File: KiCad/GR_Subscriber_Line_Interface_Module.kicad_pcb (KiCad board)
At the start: 2 copper layers, 99.3 x 99.5 mm, 112 parts, among them J1 Conn_01x03, J10 PJ-202A, J11 Screw_Terminal_01x02, J2 Conn_01x08, J3 Jumper, J4 Conn_01x06, J5 Conn_01x02, J6 RJ, J7 RJ, J8 Conn_01x03, J9 Jumper, K1 HK19F-DC5V-SHG, Q1 2N7000, Q2 2N3904, T1 600:600, U1 ESP32_DevKit_V1_DOIT, U2 MT8870DE, U3 4050, U4 KS0835F, U5 LM358, U6 LD1117AV33, U7 ICL7660, Y1 3.579545 MHz

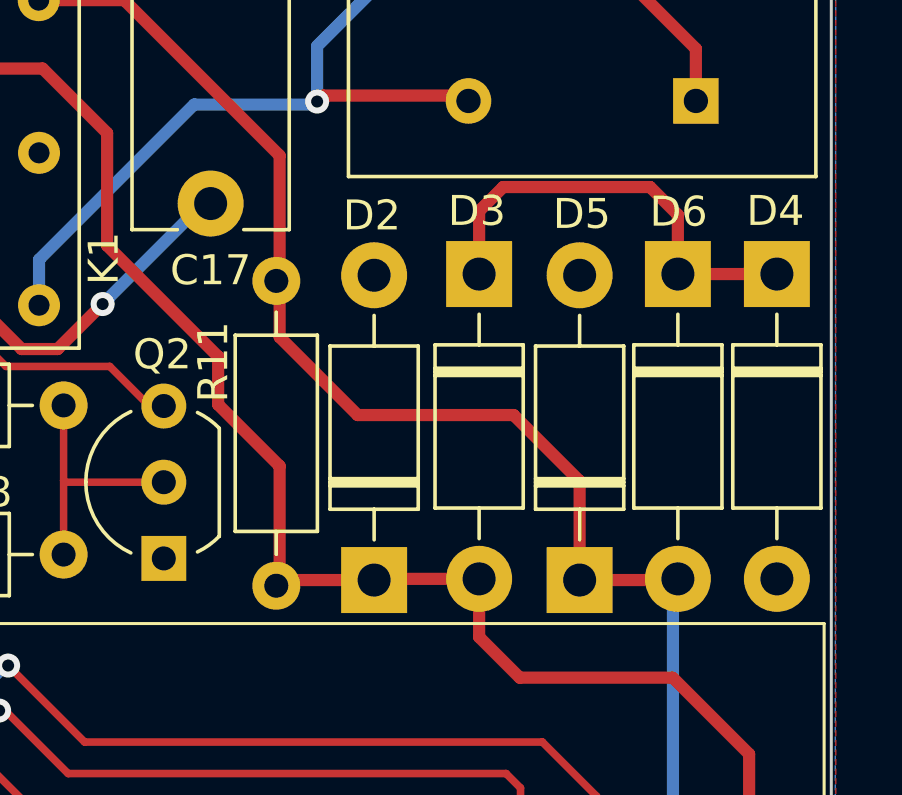
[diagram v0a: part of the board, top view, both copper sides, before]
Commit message: Add files via upload
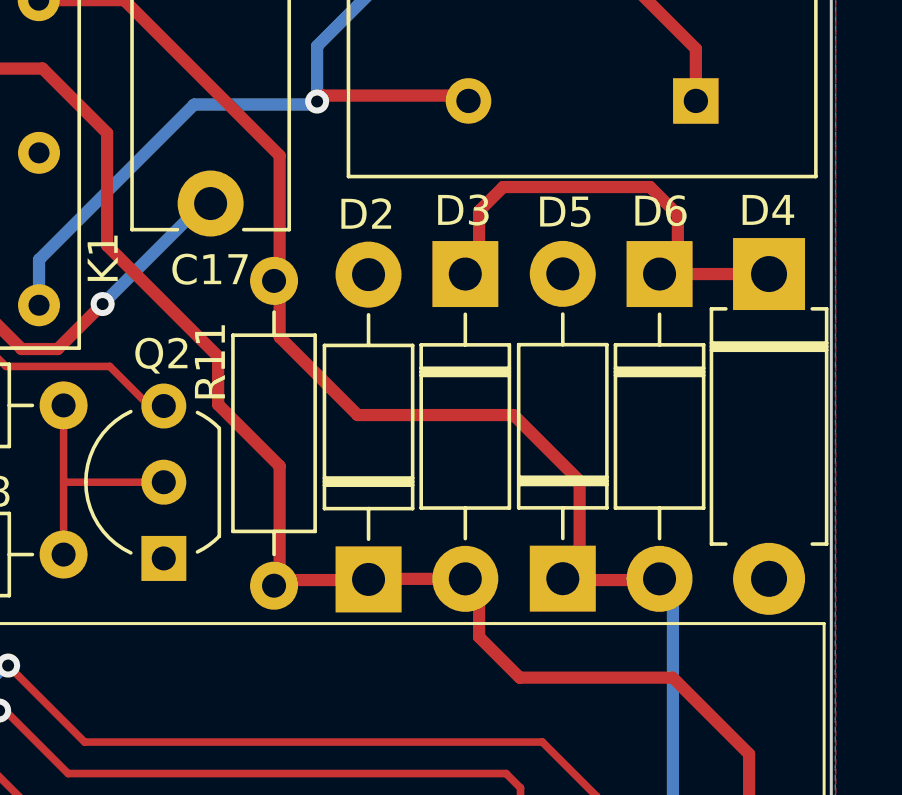
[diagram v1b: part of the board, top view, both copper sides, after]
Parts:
- D4: footprint Diode_THT:D_DO-41_SOD81_P10.16mm_Horizontal -> Diode_THT:D_DO-15_P10.16mm_Horizontal
- moved D6 0.61 mm to (200.3, 66.0)
- moved D5 0.56 mm to (197.1, 76.2)
- moved D3 0.46 mm to (193.8, 66.0)
- moved D4 0.26 mm to (203.9, 66.0)
- moved D2 0.19 mm to (190.6, 76.2)
- moved R11 0.07 mm to (187.4, 66.2)
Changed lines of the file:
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@@
     (uvia_drill 0.1)
+  )
+  (module Diode_THT:D_DO-15_P10.16mm_Horizontal (layer F.Cu)
+    (at 203.925 66.021 270)
+    (descr "Diode, DO-15 series, Axial, Horizontal, pin pitch=10.16mm, , length*diameter=7.6*3.6mm^2, , http://www.diodes.com/_files/packages/DO-15.pdf")
+    (tags "Diode DO-15 series Axial Horizontal pin pitch 10.16mm  length 7.6mm diameter 3.6mm")
+    (fp_text reference D4 (at -2.1 0.05) (layer F.SilkS)
+      (effects (font (size 1 1) (thickness 0.15)))
+    )
+    (fp_text value P6KE82 (at 5.08 2.47 90) (layer F.Fab)
+      (effects (font (size 1 1) (thickness 0.15)))
+    )
+    (fp_text user K (at 0 -2.1 90) (layer F.SilkS) hide
+      (effects (font (size 1 1) (thickness 0.15)))
+    )
+    (fp_text user K (at 0 -2.2 90) (layer F.Fab)
+      (effects (font (size 1 1) (thickness 0.15)))
+    )
+    (fp_text user %R (at 5.47 0 90) (layer F.Fab)
+      (effects (font (size 1 1) (thickness 0.15)))
+    )
+    (fp_line (start 11.61 -2.05) (end -1.45 -2.05) (layer F.CrtYd) (width 0.05))
+    (fp_line (start 11.61 2.05) (end 11.61 -2.05) (layer F.CrtYd) (width 0.05))
+    (fp_line (start -1.45 2.05) (end 11.61 2.05) (layer F.CrtYd) (width 0.05))
+    (fp_line (start -1.45 -2.05) (end -1.45 2.05) (layer F.CrtYd) (width 0.05))
+    (fp_line (start 2.3 -1.92) (end 2.3 1.92) (layer F.SilkS) (width 0.12))
+    (fp_line (start 2.54 -1.92) (end 2.54 1.92) (layer F.SilkS) (width 0.12))
+    (fp_line (start 2.42 -1.92) (end 2.42 1.92) (layer F.SilkS) (width 0.12))
+    (fp_line (start 9 1.92) (end 9 1.44) (layer F.SilkS) (width 0.12))
+    (fp_line (start 1.16 1.92) (end 9 1.92) (layer F.SilkS) (width 0.12))
+    (fp_line (start 1.16 1.44) (end 1.16 1.92) (layer F.SilkS) (width 0.12))
+    (fp_line (start 9 -1.92) (end 9 -1.44) (layer F.SilkS) (width 0.12))
+    (fp_line (start 1.16 -1.92) (end 9 -1.92) (layer F.SilkS) (width 0.12))
+    (fp_line (start 1.16 -1.44) (end 1.16 -1.92) (layer F.SilkS) (width 0.12))
+    (fp_line (start 2.32 -1.8) (end 2.32 1.8) (layer F.Fab) (width 0.1))
+    (fp_line (start 2.52 -1.8) (end 2.52 1.8) (layer F.Fab) (width 0.1))
+    (fp_line (start 2.42 -1.8) (end 2.42 1.8) (layer F.Fab) (width 0.1))
+    (fp_line (start 10.16 0) (end 8.88 0) (layer F.Fab) (width 0.1))
+    (fp_line (start 0 0) (end 1.28 0) (layer F.Fab) (width 0.1))
+    (fp_line (start 8.88 -1.8) (end 1.28 -1.8) (layer F.Fab) (width 0.1))
+    (fp_line (start 8.88 1.8) (end 8.88 -1.8) (layer F.Fab) (width 0.1))
+    (fp_line (start 1.28 1.8) (end 8.88 1.8) (layer F.Fab) (width 0.1))
+    (fp_line (start 1.28 -1.8) (end 1.28 1.8) (layer F.Fab) (width 0.1))
+    (pad 2 thru_hole oval (at 10.16 0 270) (size 2.4 2.4) (drill 1.2) (layers *.Cu *.Mask)
+      (net 1 GNDREF))
+    (pad 1 thru_hole rect (at 0 0 270) (size 2.4 2.4) (drill 1.2) (layers *.Cu *.Mask)
+      (net 41 "Net-(D3-Pad1)"))
+    (model ${KISYS3DMOD}/Diode_THT.3dshapes/D_DO-15_P10.16mm_Horizontal.wrl
+      (at (xyz 0 0 0))
+      (scale (xyz 1 1 1))
+      (rotate (xyz 0 0 0))
+    )
   )
   (module footprints:Transformer_600_600 (layer F.Cu)
@@
   )
   (module Resistor_THT:R_Axial_DIN0207_L6.3mm_D2.5mm_P10.16mm_Horizontal (layer F.Cu)
-    (at 187.5 66.25 270)
+    (at 187.425 66.25 270)
     (descr "Resistor, Axial_DIN0207 series, Axial, Horizontal, pin pitch=10.16mm, 0.25W = 1/4W, length*diameter=6.3*2.5mm^2, http://cdn-reichelt.de/documents/datenblatt/B400/1_4W%23YAG.pdf")
     (tags "Resistor Axial_DIN0207 series Axial Horizontal pin pitch 10.16mm 0.25W = 1/4W length 6.3mm diameter 2.5mm")
@@
   )
   (module Diode_THT:D_DO-41_SOD81_P10.16mm_Horizontal (layer F.Cu)
-    (at 190.761 76.221 90)
+    (at 190.575 76.2 90)
     (descr "Diode, DO-41_SOD81 series, Axial, Horizontal, pin pitch=10.16mm, , length*diameter=5.2*2.7mm^2, , http://www.diodes.com/_files/packages/DO-41%20(Plastic).pdf")
     (tags "Diode DO-41_SOD81 series Axial Horizontal pin pitch 10.16mm  length 5.2mm diameter 2.7mm")
@@
   )
   (module Diode_THT:D_DO-41_SOD81_P10.16mm_Horizontal (layer F.Cu)
-    (at 194.261 66.021 270)
+    (at 193.8 66.021 270)
     (descr "Diode, DO-41_SOD81 series, Axial, Horizontal, pin pitch=10.16mm, , length*diameter=5.2*2.7mm^2, , http://www.diodes.com/_files/packages/DO-41%20(Plastic).pdf")
     (tags "Diode DO-41_SOD81 series Axial Horizontal pin pitch 10.16mm  length 5.2mm diameter 2.7mm")
@@
   )
   (module Diode_THT:D_DO-41_SOD81_P10.16mm_Horizontal (layer F.Cu)
-    (at 204.186 66.021 270)
+    (at 197.05 76.175 90)
     (descr "Diode, DO-41_SOD81 series, Axial, Horizontal, pin pitch=10.16mm, , length*diameter=5.2*2.7mm^2, , http://www.diodes.com/_files/packages/DO-41%20(Plastic).pdf")
     (tags "Diode DO-41_SOD81 series Axial Horizontal pin pitch 10.16mm  length 5.2mm diameter 2.7mm")
-    (fp_text reference D4 (at -2.1 0.05) (layer F.SilkS)
-      (effects (font (size 1 1) (thickness 0.15)))
-    )
-    (fp_text value P6KE82 (at 5.08 2.47 90) (layer F.Fab)
+    (fp_text reference D5 (at 12.2 0.075) (layer F.SilkS)
+      (effects (font (size 1 1) (thickness 0.15)))
+    )
+    (fp_text value 1N4004 (at 5.08 2.47 90) (layer F.Fab)
       (effects (font (size 1 1) (thickness 0.15)))
     )
@@
       (effects (font (size 1 1) (thickness 0.15)))
     )
-    (pad 1 thru_hole rect (at 0 0 270) (size 2.2 2.2) (drill 1.1) (layers *.Cu *.Mask)
-      (net 41 "Net-(D3-Pad1)"))
-    (pad 2 thru_hole oval (at 10.16 0 270) (size 2.2 2.2) (drill 1.1) (layers *.Cu *.Mask)
-      (net 1 GNDREF))
-    (model ${KISYS3DMOD}/Diode_THT.3dshapes/D_DO-41_SOD81_P10.16mm_Horizontal.wrl
-      (at (xyz 0 0 0))
-      (scale (xyz 1 1 1))
-      (rotate (xyz 0 0 0))
-    )
-  )
-  (module Diode_THT:D_DO-41_SOD81_P10.16mm_Horizontal (layer F.Cu)
-    (at 197.611 76.221 90)
-    (descr "Diode, DO-41_SOD81 series, Axial, Horizontal, pin pitch=10.16mm, , length*diameter=5.2*2.7mm^2, , http://www.diodes.com/_files/packages/DO-41%20(Plastic).pdf")
-    (tags "Diode DO-41_SOD81 series Axial Horizontal pin pitch 10.16mm  length 5.2mm diameter 2.7mm")
-    (fp_text reference D5 (at 12.2 0.075) (layer F.SilkS)
-      (effects (font (size 1 1) (thickness 0.15)))
-    )
-    (fp_text value 1N4004 (at 5.08 2.47 90) (layer F.Fab)
-      (effects (font (size 1 1) (thickness 0.15)))
-    )
-    (fp_line (start 2.48 -1.35) (end 2.48 1.35) (layer F.Fab) (width 0.1))
-    (fp_line (start 2.48 1.35) (end 7.68 1.35) (layer F.Fab) (width 0.1))
-    (fp_line (start 7.68 1.35) (end 7.68 -1.35) (layer F.Fab) (width 0.1))
-    (fp_line (start 7.68 -1.35) (end 2.48 -1.35) (layer F.Fab) (width 0.1))
-    (fp_line (start 0 0) (end 2.48 0) (layer F.Fab) (width 0.1))
-    (fp_line (start 10.16 0) (end 7.68 0) (layer F.Fab) (width 0.1))
-    (fp_line (start 3.26 -1.35) (end 3.26 1.35) (layer F.Fab) (width 0.1))
-    (fp_line (start 3.36 -1.35) (end 3.36 1.35) (layer F.Fab) (width 0.1))
-    (fp_line (start 3.16 -1.35) (end 3.16 1.35) (layer F.Fab) (width 0.1))
-    (fp_line (start 2.36 -1.47) (end 2.36 1.47) (layer F.SilkS) (width 0.12))
-    (fp_line (start 2.36 1.47) (end 7.8 1.47) (layer F.SilkS) (width 0.12))
-    (fp_line (start 7.8 1.47) (end 7.8 -1.47) (layer F.SilkS) (width 0.12))
-    (fp_line (start 7.8 -1.47) (end 2.36 -1.47) (layer F.SilkS) (width 0.12))
-    (fp_line (start 1.34 0) (end 2.36 0) (layer F.SilkS) (width 0.12))
-    (fp_line (start 8.82 0) (end 7.8 0) (layer F.SilkS) (width 0.12))
-    (fp_line (start 3.26 -1.47) (end 3.26 1.47) (layer F.SilkS) (width 0.12))
-    (fp_line (start 3.38 -1.47) (end 3.38 1.47) (layer F.SilkS) (width 0.12))
-    (fp_line (start 3.14 -1.47) (end 3.14 1.47) (layer F.SilkS) (width 0.12))
-    (fp_line (start -1.35 -1.6) (end -1.35 1.6) (layer F.CrtYd) (width 0.05))
-    (fp_line (start -1.35 1.6) (end 11.51 1.6) (layer F.CrtYd) (width 0.05))
-    (fp_line (start 11.51 1.6) (end 11.51 -1.6) (layer F.CrtYd) (width 0.05))
-    (fp_line (start 11.51 -1.6) (end -1.35 -1.6) (layer F.CrtYd) (width 0.05))
-    (fp_text user %R (at 5.47 0 90) (layer F.Fab)
-      (effects (font (size 1 1) (thickness 0.15)))
-    )
-    (fp_text user K (at 0 -2.1 90) (layer F.Fab)
-      (effects (font (size 1 1) (thickness 0.15)))
-    )
-    (fp_text user K (at 0 -2.1 90) (layer F.SilkS) hide
-      (effects (font (size 1 1) (thickness 0.15)))
-    )
     (pad 1 thru_hole rect (at 0 0 90) (size 2.2 2.2) (drill 1.1) (layers *.Cu *.Mask)
       (net 42 "/KS0835F SLIC/Tip"))
@@
   )
   (module Diode_THT:D_DO-41_SOD81_P10.16mm_Horizontal (layer F.Cu)
-    (at 200.886001 66.021 270)
+    (at 200.275 66.021 270)
     (descr "Diode, DO-41_SOD81 series, Axial, Horizontal, pin pitch=10.16mm, , length*diameter=5.2*2.7mm^2, , http://www.diodes.com/_files/packages/DO-41%20(Plastic).pdf")
     (tags "Diode DO-41_SOD81 series Axial Horizontal pin pitch 10.16mm  length 5.2mm diameter 2.7mm")
